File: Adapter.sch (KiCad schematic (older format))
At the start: 19 parts, among them J1 PSU_CONNECTOR, J10 12V, J11 12V, J12 RTN, J13 RTN, J14 RTN, J2 CONN_01X03, J3 PEG, J4 PEG, J5 PEG, J6 PEG, J7 PEG, J8 PEG, J9 12V, SW1 SW_SPST

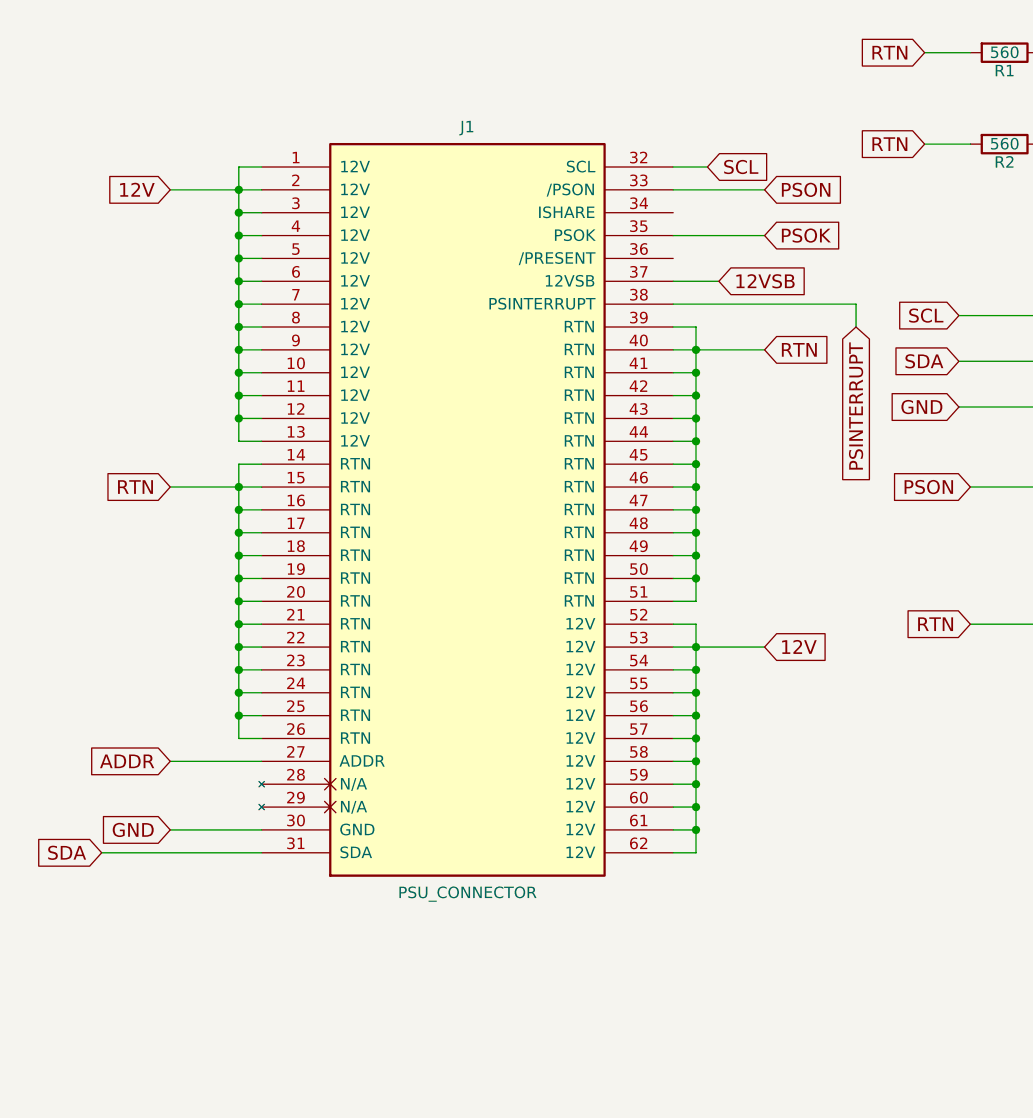
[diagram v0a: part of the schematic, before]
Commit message: Further layout work.
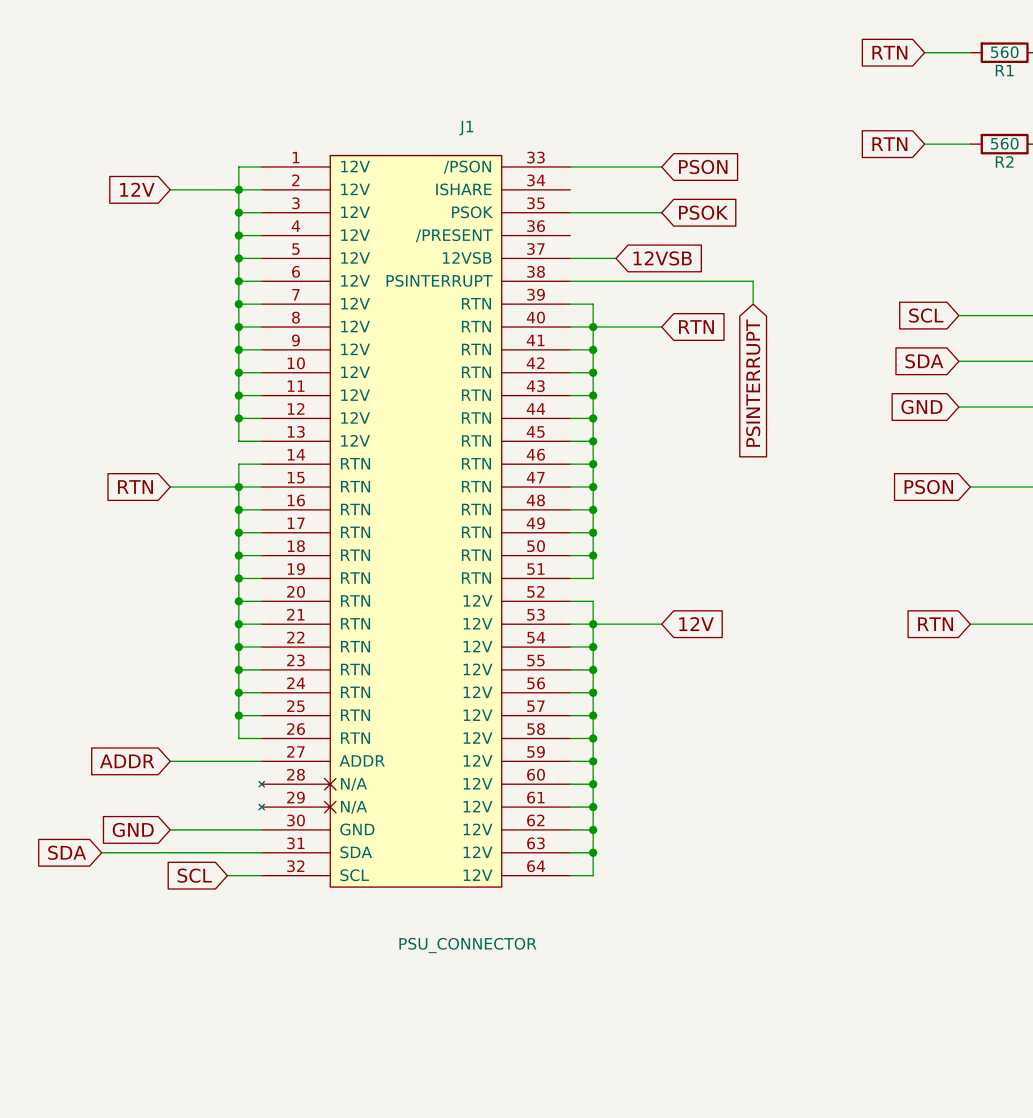
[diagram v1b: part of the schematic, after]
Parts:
- removed J1: PSU_CONNECTOR, psu_connector:COMMON_SLOT_PSU, symbol PSU_CONNECTOR-RESCUE-Adapter
- added J1: PSU_CONNECTOR, psu_connector:COMMON_SLOT_PSU, symbol PSU_CONNECTOR
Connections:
- net 12V: now also J1.1 (12V), J1.10 (12V), J1.11 (12V), J1.12 (12V), J1.13 (12V), J1.2 (12V), J1.3 (12V), J1.4 (12V), J1.5 (12V), J1.52 (12V), J1.53 (12V), J1.54 (12V), J1.55 (12V), J1.56 (12V), J1.57 (12V), J1.58 (12V), J1.59 (12V), J1.6 (12V), J1.60 (12V), J1.61 (12V), J1.62 (12V), J1.63 (12V), J1.64 (12V), J1.7 (12V), J1.8 (12V), J1.9 (12V)
- net 12VSB: now also J1.37 (12VSB)
- net ADDR: now also J1.27 (ADDR)
- net GND: now also J1.30 (GND)
- net PSINTERRUPT: now also J1.38 (PSINTERRUPT)
- net PSOK: now also J1.35 (PSOK)
- net PSON: now also J1.33 (/PSON)
- net RTN: now also J1.14 (RTN), J1.15 (RTN), J1.16 (RTN), J1.17 (RTN), J1.18 (RTN), J1.19 (RTN), J1.20 (RTN), J1.21 (RTN), J1.22 (RTN), J1.23 (RTN), J1.24 (RTN), J1.25 (RTN), J1.26 (RTN), J1.39 (RTN), J1.40 (RTN), J1.41 (RTN), J1.42 (RTN), J1.43 (RTN), J1.44 (RTN), J1.45 (RTN), J1.46 (RTN), J1.47 (RTN), J1.48 (RTN), J1.49 (RTN), J1.50 (RTN), J1.51 (RTN)
- net SCL: now also J1.32 (SCL)
- net SDA: now also J1.31 (SDA)
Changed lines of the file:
@@
 Comment4 ""
 $EndDescr
-Text GLabel 3900 4200 2    60   Input ~ 0
+Text GLabel 3450 4100 2    60   Input ~ 0
 12V
 Text GLabel 1300 2200 0    60   Input ~ 0
@@
 Text GLabel 1300 3500 0    60   Input ~ 0
 RTN
-Text GLabel 3900 2900 2    60   Input ~ 0
+Text GLabel 3450 2800 2    60   Input ~ 0
 RTN
-Text GLabel 3700 2600 2    60   Input ~ 0
+Text GLabel 3250 2500 2    60   Input ~ 0
 12VSB
-Text GLabel 4300 2800 3    60   Input ~ 0
+Text GLabel 3850 2700 3    60   Input ~ 0
 PSINTERRUPT
-Text GLabel 3650 2100 2    60   Input ~ 0
+Text GLabel 1550 5200 0    60   Input ~ 0
 SCL
 Text GLabel 1000 5100 0    60   Input ~ 0
 SDA
-Text GLabel 3900 2200 2    60   Input ~ 0
+Text GLabel 3450 2100 2    60   Input ~ 0
 PSON
 Text GLabel 1300 4700 0    60   Input ~ 0
@@
 Text GLabel 1300 5000 0    60   Input ~ 0
 GND
-Text GLabel 3900 2400 2    60   Input ~ 0
+Text GLabel 3450 2300 2    60   Input ~ 0
 PSOK
 $Comp
@@
 	0    1    1    0
 $EndComp
-$Comp
-L PSU_CONNECTOR-RESCUE-Adapter J1
-U 1 1 5949B0F8
-P 2600 3600
-F 0 "J1" H 2600 5275 50  0000 C CNN
-F 1 "PSU_CONNECTOR" H 2600 1925 50  0000 C CNN
-F 2 "psu_connector:COMMON_SLOT_PSU" H 2600 3600 50  0001 C CNN
-F 3 "" H 2600 3600 50  0001 C CNN
-	1    2600 3600
-	1    0    0    -1
-$EndComp
 Wire Wire Line
 	4600 1600 4800 1600
@@
 Connection ~ 1600 3500
 Wire Wire Line
-	3500 2800 3600 2800
-Wire Wire Line
-	3600 2800 3600 4000
-Wire Wire Line
-	3600 4000 3500 4000
-Wire Wire Line
-	3500 4100 3600 4100
-Wire Wire Line
-	3600 4100 3600 5100
-Wire Wire Line
-	3600 5100 3500 5100
-Wire Wire Line
-	3500 2900 3900 2900
-Connection ~ 3600 2900
-Wire Wire Line
-	3500 3000 3600 3000
-Connection ~ 3600 3000
-Wire Wire Line
-	3500 3100 3600 3100
-Connection ~ 3600 3100
-Wire Wire Line
-	3500 3200 3600 3200
-Connection ~ 3600 3200
-Wire Wire Line
-	3500 3300 3600 3300
-Connection ~ 3600 3300
-Wire Wire Line
-	3500 3400 3600 3400
-Connection ~ 3600 3400
-Wire Wire Line
-	3500 3500 3600 3500
-Connection ~ 3600 3500
-Wire Wire Line
-	3500 3600 3600 3600
-Connection ~ 3600 3600
-Wire Wire Line
-	3500 3700 3600 3700
-Connection ~ 3600 3700
-Wire Wire Line
-	3500 3800 3600 3800
-Connection ~ 3600 3800
-Wire Wire Line
-	3500 3900 3600 3900
-Connection ~ 3600 3900
-Wire Wire Line
-	3500 4200 3900 4200
-Connection ~ 3600 4200
-Wire Wire Line
-	3500 4300 3600 4300
-Connection ~ 3600 4300
-Wire Wire Line
-	3500 4400 3600 4400
-Connection ~ 3600 4400
-Wire Wire Line
-	3500 4500 3600 4500
-Connection ~ 3600 4500
-Wire Wire Line
-	3500 4600 3600 4600
-Connection ~ 3600 4600
-Wire Wire Line
-	3500 4700 3600 4700
-Connection ~ 3600 4700
-Wire Wire Line
-	3500 4800 3600 4800
-Connection ~ 3600 4800
-Wire Wire Line
-	3500 4900 3600 4900
-Connection ~ 3600 4900
-Wire Wire Line
-	3500 5000 3600 5000
-Connection ~ 3600 5000
+	3050 2700 3150 2700
+Wire Wire Line
+	3150 2700 3150 3900
+Wire Wire Line
+	3150 3900 3050 3900
+Wire Wire Line
+	3050 4000 3150 4000
+Wire Wire Line
+	3150 4000 3150 5200
+Wire Wire Line
+	3150 5000 3050 5000
+Wire Wire Line
+	3050 2800 3450 2800
+Connection ~ 3150 2800
+Wire Wire Line
+	3050 2900 3150 2900
+Connection ~ 3150 2900
+Wire Wire Line
+	3050 3000 3150 3000
+Connection ~ 3150 3000
+Wire Wire Line
+	3050 3100 3150 3100
+Connection ~ 3150 3100
+Wire Wire Line
+	3050 3200 3150 3200
+Connection ~ 3150 3200
+Wire Wire Line
+	3050 3300 3150 3300
+Connection ~ 3150 3300
+Wire Wire Line
+	3050 3400 3150 3400
+Connection ~ 3150 3400
+Wire Wire Line
+	3050 3500 3150 3500
+Connection ~ 3150 3500
+Wire Wire Line
+	3050 3600 3150 3600
+Connection ~ 3150 3600
+Wire Wire Line
+	3050 3700 3150 3700
+Connection ~ 3150 3700
+Wire Wire Line
+	3050 3800 3150 3800
+Connection ~ 3150 3800
+Wire Wire Line
+	3050 4100 3450 4100
+Connection ~ 3150 4100
+Wire Wire Line
+	3050 4200 3150 4200
+Connection ~ 3150 4200
+Wire Wire Line
+	3050 4300 3150 4300
+Connection ~ 3150 4300
+Wire Wire Line
+	3050 4400 3150 4400
+Connection ~ 3150 4400
+Wire Wire Line
+	3050 4500 3150 4500
+Connection ~ 3150 4500
+Wire Wire Line
+	3050 4600 3150 4600
+Connection ~ 3150 4600
+Wire Wire Line
+	3050 4700 3150 4700
+Connection ~ 3150 4700
+Wire Wire Line
+	3050 4800 3150 4800
+Connection ~ 3150 4800
+Wire Wire Line
+	3050 4900 3150 4900
+Connection ~ 3150 4900
 Wire Wire Line
 	1700 4700 1300 4700
@@
 	1000 5100 1700 5100
 Wire Wire Line
-	3650 2100 3500 2100
-Wire Wire Line
-	3500 2200 3900 2200
-Wire Wire Line
-	3500 2400 3900 2400
-Wire Wire Line
-	3700 2600 3500 2600
-Wire Wire Line
-	3500 2700 4300 2700
-Wire Wire Line
-	4300 2700 4300 2800
+	3050 2100 3450 2100
+Wire Wire Line
+	3050 2300 3450 2300
+Wire Wire Line
+	3250 2500 3050 2500
+Wire Wire Line
+	3050 2600 3850 2600
+Wire Wire Line
+	3850 2600 3850 2700
 $Comp
 L CONN_01X03 J9
@@
 	2200 7100 2200 6900
 Connection ~ 2200 6900
+$Comp
+L PSU_CONNECTOR J1
+U 1 1 594BC644
+P 2600 3600
+F 0 "J1" H 2600 5275 50  0000 C CNN
+F 1 "PSU_CONNECTOR" H 2600 1700 50  0000 C CNN
+F 2 "psu_connector:COMMON_SLOT_PSU" H 2150 3600 50  0001 C CNN
+F 3 "" H 2150 3600 50  0001 C CNN
+	1    2600 3600
+	1    0    0    -1
+$EndComp
+Wire Wire Line
+	3150 5200 3050 5200
+Connection ~ 3150 5000
+Wire Wire Line
+	3050 5100 3150 5100
+Connection ~ 3150 5100
+Wire Wire Line
+	1550 5200 1700 5200
 $EndSCHEMATC
